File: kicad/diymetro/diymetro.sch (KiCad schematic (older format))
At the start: 32 parts, among them J1 AudioJack2_SwitchT, J2 AudioJack2_SwitchT, J3 AudioJack2_SwitchT, J4 AudioJack2_SwitchT, J5 Conn_02x08_Top_Bottom, J6 AudioJack2_SwitchT, J7 ICSP, J8 SER, Q1 MMBT2222A, Q2 MMBT2222A, SW10 SW_Push, U5 ATmega328P-PU, Y1 Crystal

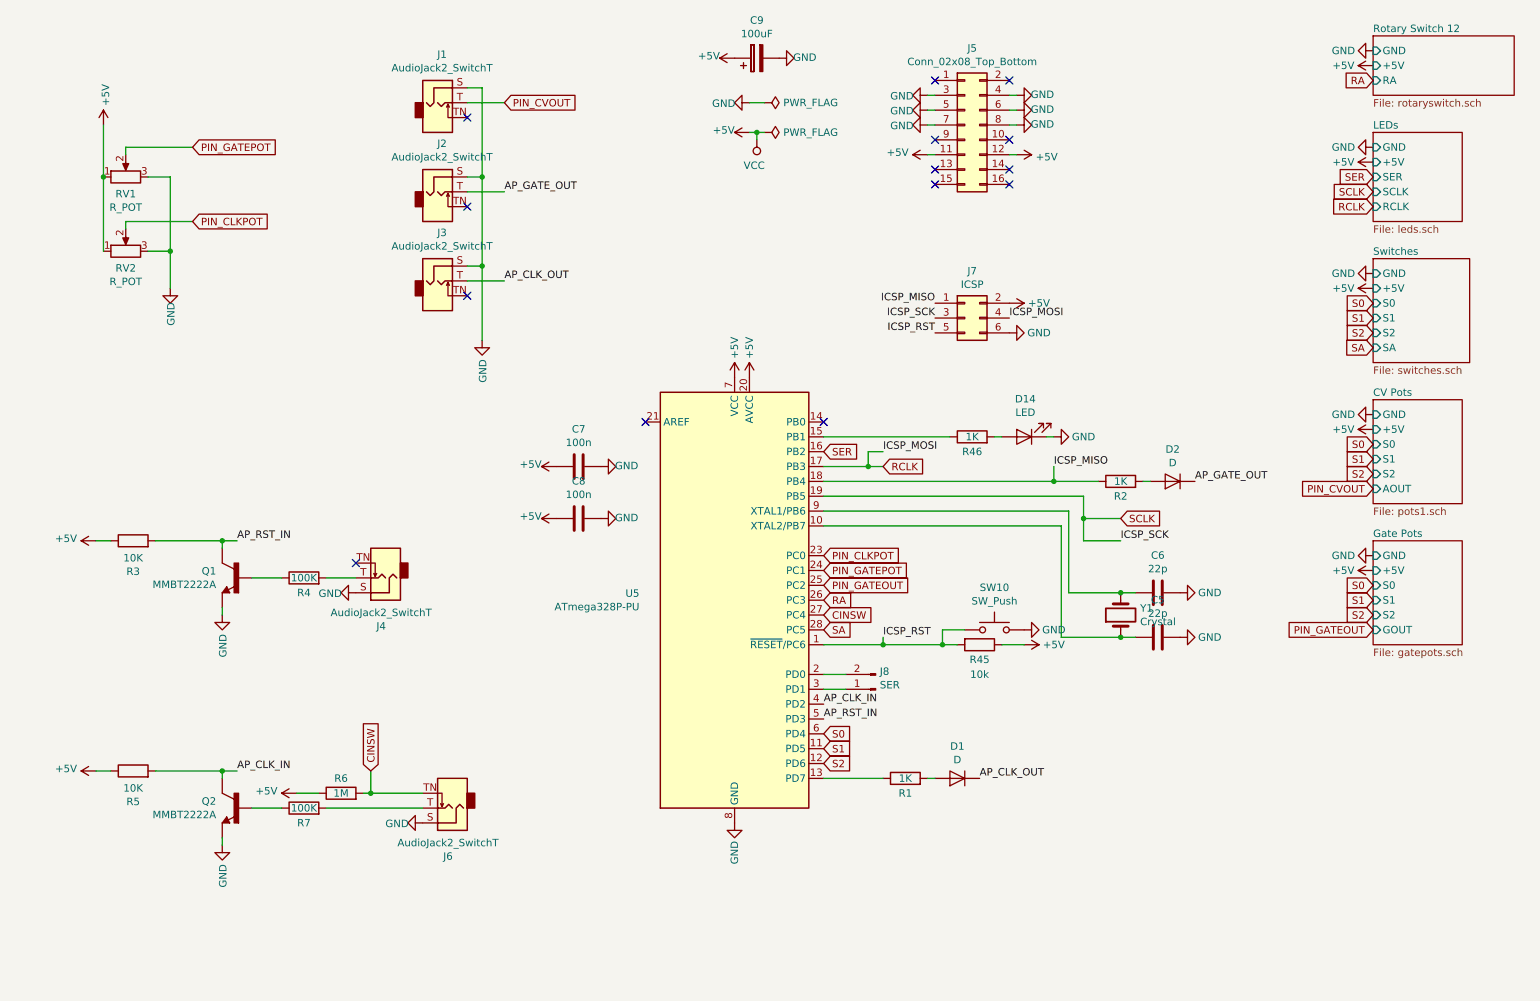
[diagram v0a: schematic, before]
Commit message: Add TL072 output buffers for gate/clock/cv outputs.
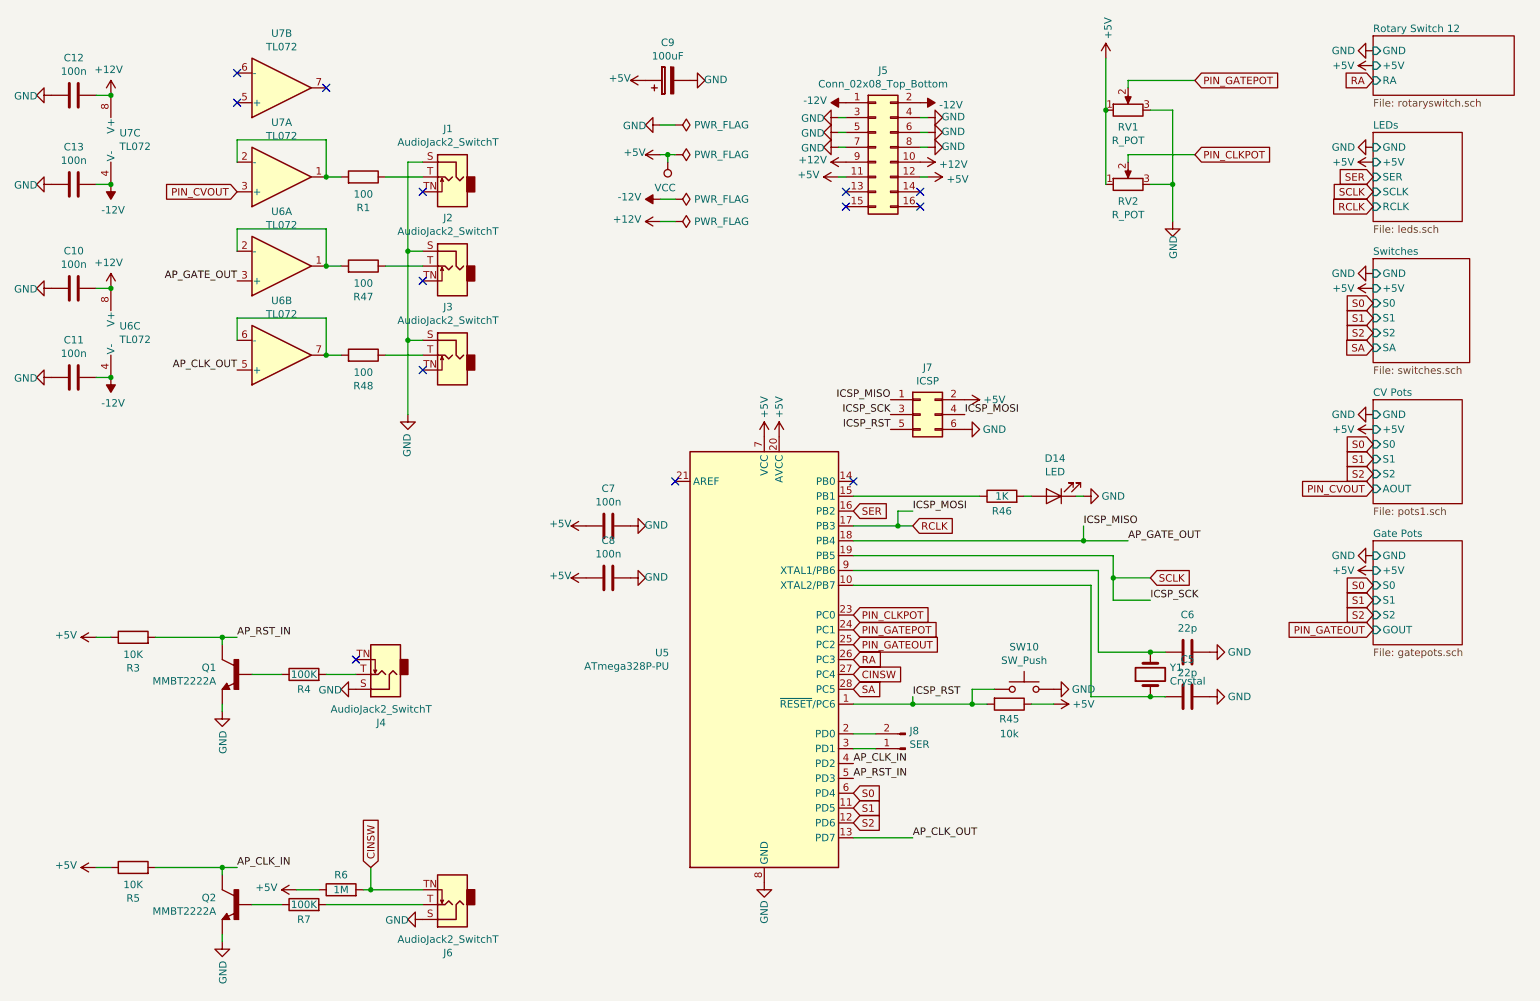
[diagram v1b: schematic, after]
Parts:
- removed D1, D2: D, Diode_SMD:D_1206_3216Metric, symbol Device:D
- removed R2: 1K, Resistor_SMD:R_1206_3216Metric, symbol Device:R
- added C10, C11, C12, C13: 100n, Capacitor_SMD:C_1206_3216Metric, symbol Device:C
- added R47, R48: 100, Resistor_SMD:R_1206_3216Metric, symbol Device:R
- added U6, U7: TL072, Package_SO:SO-8_5.3x6.2mm_P1.27mm, symbol Amplifier_Operational:TL072
- R1: value 1K -> 100
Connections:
- net ICSP_MISO is gone; now on net AP_GATE_OUT: J7.1 (Pin_1), U5.18 (PB4)
- net AP_CLK_OUT: now also U5.13 (PD7), U6.5 (+); no longer J3.T
- net AP_GATE_OUT: now also U6.3 (+); no longer J2.T
- net GND: now also C10.1, C11.1, C12.1, C13.1
- net PIN_CVOUT: now also U7.3 (+); no longer J1.T
- net -12V: now reaches J5.1 (Pin_1)
- net -12V: now also J5.2 (Pin_2), C11.2, C13.2, U6.4 (V-), U7.4 (V-)
- net +12V: now reaches J5.10 (Pin_10)
- net +12V: now also J5.9 (Pin_9), C10.2, C12.2, U6.8 (V+), U7.8 (V+)
- net at R1.1: now also J1.T; no longer U5.13 (PD7)
- net at R1.2: now also U7.1, U7.2 (-)
- new net: J2.T, R47.1
- new net: J3.T, R48.1
- new net: R47.2, U6.1, U6.2 (-)
- new net: R48.2, U6.6 (-), U6.7
- no-connect marks 14 -> 13
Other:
- moved on the sheet: C5, C6, C7, C8, C9, D14, J1, J2, J3, J4, J5, J6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
